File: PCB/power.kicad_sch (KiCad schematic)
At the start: 40 parts, among them U2 MAX20029ATIA/V+, U5 TPS2121RUXR

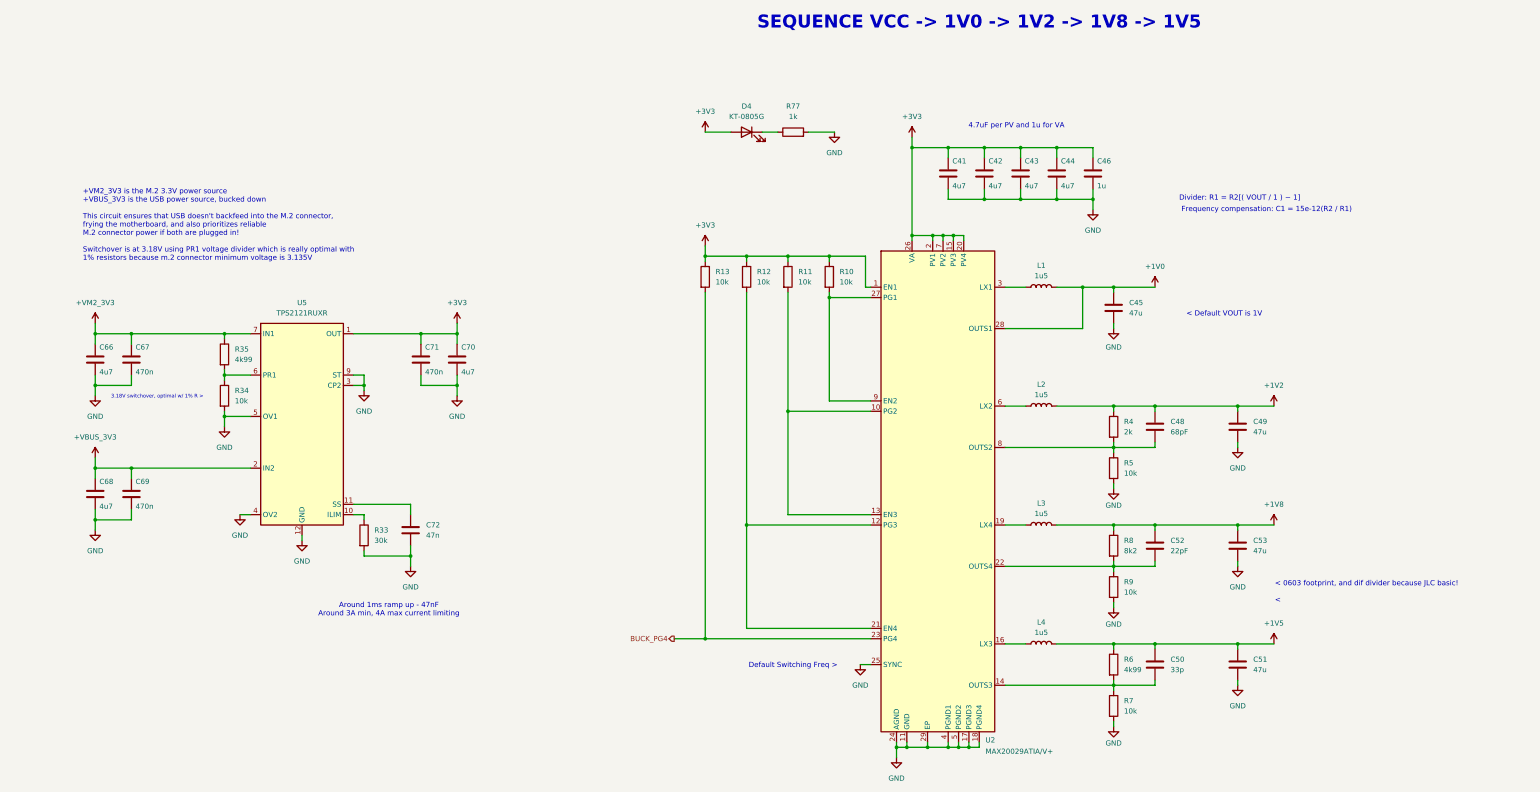
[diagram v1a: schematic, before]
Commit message: adding return via's and cleaning up the schematic a bit!
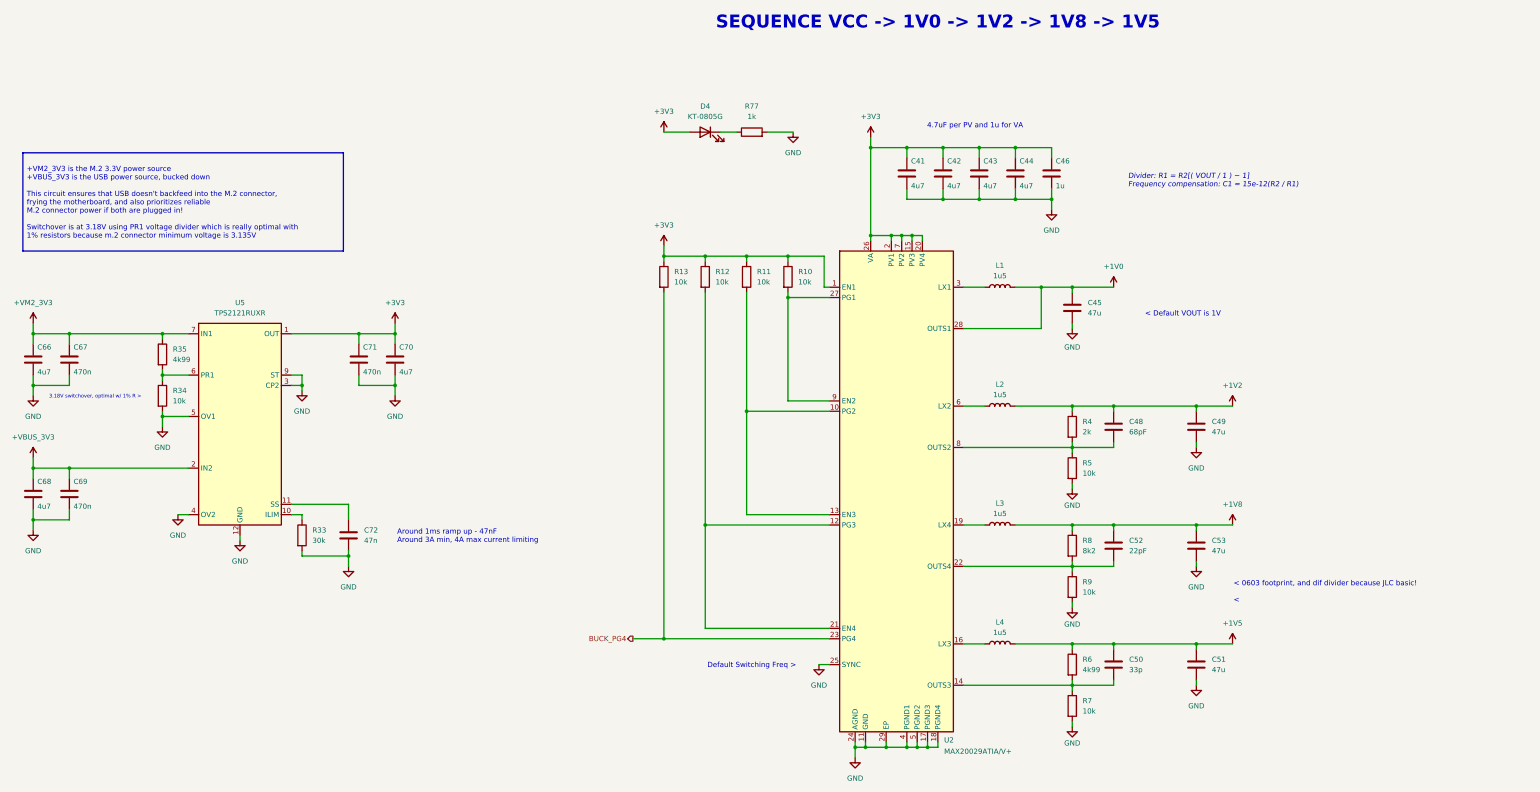
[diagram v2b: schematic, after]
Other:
- note added: "Divider: R1 = R2[( VOUT / 1 ) − 1] Frequency compensation: C1 = 15e-12(R2 / R1)"
- note removed: "+VM2_3V3 is the M.2 3.3V power source +VBUS_3V3 is the USB power source, bucked down This circuit ensures that USB doesn't backfeed into the M.2 connector, frying the motherboard, and also prioritizes reliable M.2 connector power if both are plugged in! Switchover is at 3.18V using PR1 voltage divider which is really optimal with 1% resistors because m.2 connector minimum voltage is 3.135V"
- note removed: "Divider: R1 = R2[( VOUT / 1 ) − 1]"
- note removed: "Frequency compensation: C1 = 15e-12(R2 / R1)"
- moved on the sheet: C41, C42, C43, C44, C45, C46, C48, C49, C50, C51, C52, C53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
